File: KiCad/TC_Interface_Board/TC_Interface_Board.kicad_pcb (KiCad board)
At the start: 2 copper layers, 68.9 x 121.6 mm, 30 parts, among them J1 JST_VH_01x05, J1_24V1 JST_VH_01x04, J1_CN1 JST_VH_01x03, J2 JST_VH_01x05, J2_CN1 JST_VH_01x02, J3 JST_VH_01x05, J3_CN1 JST_VH_01x02, J4 JST_VH_01x05, J5 JST_VH_01x05, J6 JST_VH_01x05, J7 JST_VH_01x05, J8 JST_VH_01x05, Q1 DTC143E, Q2 DTC143E, U1 MC34063AP

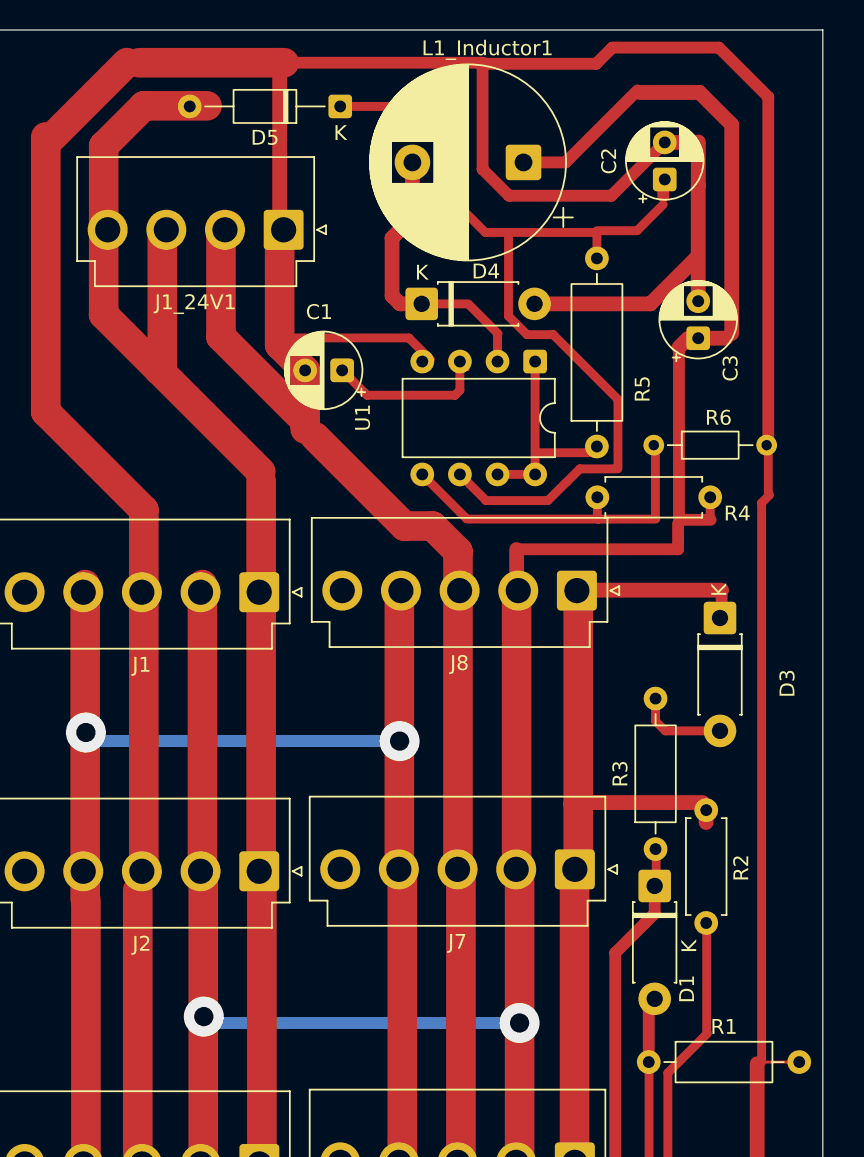
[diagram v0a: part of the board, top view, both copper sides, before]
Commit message: UPDATE
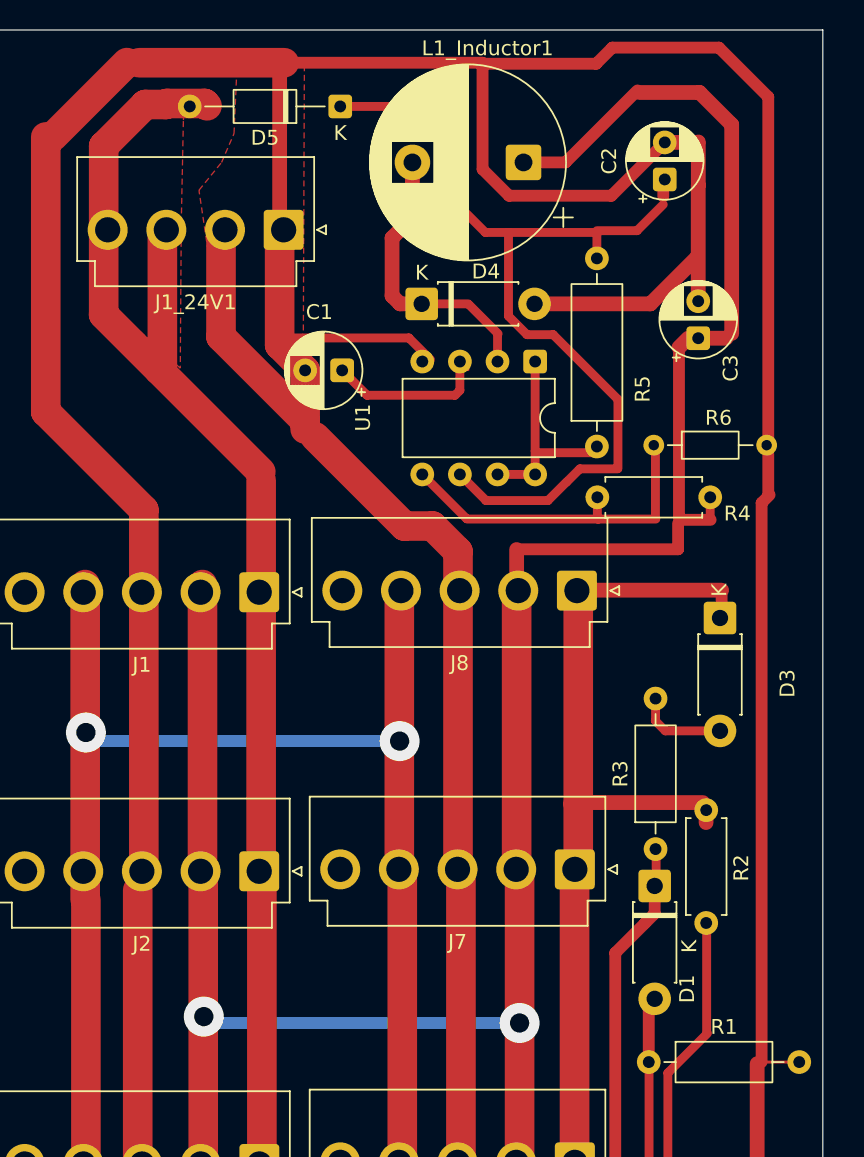
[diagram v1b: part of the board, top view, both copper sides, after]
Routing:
- added copper zone on F.Cu, net +24V
- added copper zone on F.Cu, net GND
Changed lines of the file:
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@@
+	)
+	(segment
+		(start 135.96 37.09)
+		(end 136.12 37.25)
+		(width 2)
+		(layer "F.Cu")
+		(net 1)
 	)
 	(segment
@@
 	)
 	(segment
+		(start 129.14 39.97)
+		(end 131.95 37.16)
+		(width 2)
+		(layer "F.Cu")
+		(net 1)
+	)
+	(segment
 		(start 169.81 85.64)
 		(end 169.81 84.51)
@@
 	)
 	(segment
-		(start 129.14 45.72)
-		(end 129.14 39.97)
-		(width 2)
-		(layer "F.Cu")
-		(net 1)
-	)
-	(segment
 		(start 161.2 69.95)
 		(end 160.98 70.17)
@@
 	)
 	(segment
-		(start 131.86 37.25)
-		(end 136.12 37.25)
+		(start 129.14 51.33)
+		(end 129.14 39.97)
+		(width 2)
+		(layer "F.Cu")
+		(net 1)
+	)
+	(segment
+		(start 133.41 37.09)
+		(end 135.96 37.09)
 		(width 2)
 		(layer "F.Cu")
@@
 	)
 	(segment
+		(start 131.95 37.16)
+		(end 133.34 37.16)
+		(width 2)
+		(layer "F.Cu")
+		(net 1)
+	)
+	(segment
+		(start 133.34 37.16)
+		(end 133.41 37.09)
+		(width 2)
+		(layer "F.Cu")
+		(net 1)
+	)
+	(segment
 		(start 139.77 62.54)
 		(end 139.75 62.52)
@@
 	)
 	(segment
-		(start 129.14 51.33)
-		(end 129.14 45.72)
-		(width 2)
-		(layer "F.Cu")
-		(net 1)
-	)
-	(segment
 		(start 132.87 55.08)
 		(end 129.13 51.34)
@@
 	)
 	(segment
-		(start 129.14 39.97)
-		(end 131.86 37.25)
-		(width 2)
-		(layer "F.Cu")
-		(net 1)
-	)
-	(segment
 		(start 161.096428 133.96)
 		(end 161.2 133.856428)
@@
 		(start 174.01 63.43)
 		(end 174.01 60.771)
-		(width 0.6)
+		(width 0.8)
 		(layer "F.Cu")
 		(net 4)
@@
 		(start 173.56 101.81)
 		(end 173.56 64.06)
-		(width 0.6)
+		(width 0.8)
 		(layer "F.Cu")
 		(net 4)
@@
 		(start 173.56 64.06)
 		(end 174.1 63.52)
-		(width 0.6)
+		(width 0.8)
 		(layer "F.Cu")
 		(net 4)
@@
 		(net 21)
 	)
+	(zone
+		(net 4)
+		(net_name "GND")
+		(layer "F.Cu")
+		(hatch edge 0.5)
+		(priority 1)
+		(connect_pads
+			(clearance 0.5)
+		)
+		(min_thickness 0.25)
+		(filled_areas_thickness no)
+		(fill yes
+			(thermal_gap 0.5)
+			(thermal_bridge_width 0.5)
+		)
+		(polygon
+			(pts
+				(xy 142.69 34.51) (xy 142.62 52.65) (xy 141.43 53.35) (xy 142.06 56.49) (xy 137.06 52.84) (xy 135.5725 42.95)
+				(xy 137.1 41.07) (xy 137.94 39.12) (xy 138.15 34.37) (xy 142.83 34.51)
+			)
+		)
+	)
+	(zone
+		(net 1)
+		(net_name "+24V")
+		(layer "F.Cu")
+		(hatch edge 0.5)
+		(connect_pads
+			(clearance 0.5)
+		)
+		(min_thickness 0.25)
+		(filled_areas_thickness no)
+		(fill yes
+			(thermal_gap 0.5)
+			(thermal_bridge_width 0.5)
+		)
+		(polygon
+			(pts
+				(xy 134.52 38.28) (xy 134.38 45.07) (xy 134.31 54.96) (xy 129.71 50.77) (xy 129.78 40.16) (xy 132.43 37.93)
+				(xy 134.59 37.16)
+			)
+		)
+	)
 	(embedded_fonts no)

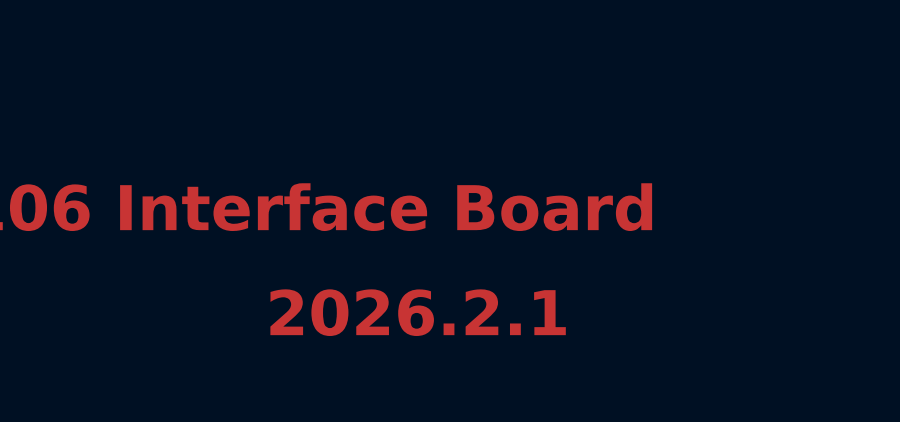
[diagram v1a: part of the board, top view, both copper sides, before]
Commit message: UPDATE
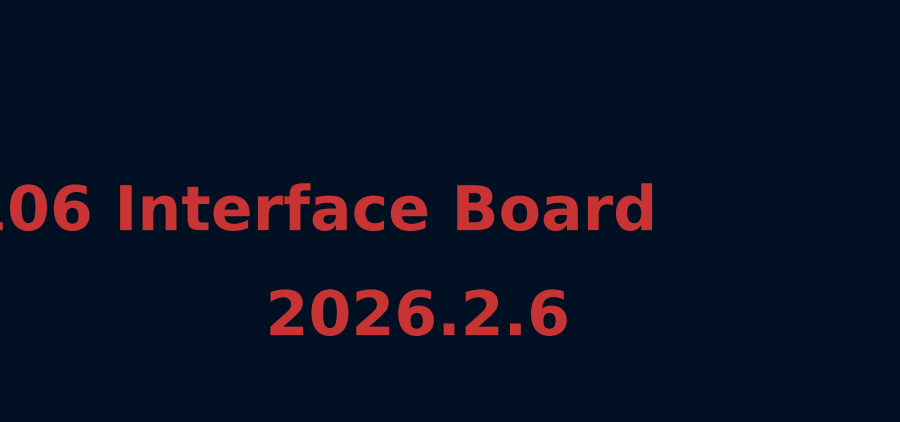
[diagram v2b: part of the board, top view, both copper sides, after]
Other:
- board text added: "2026.2.6"
- board text removed: "2026.2.1"
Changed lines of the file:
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@@
 		)
 	)
-	(gr_text "2026.2.1"
+	(gr_text "2026.2.6"
 		(at 212 194 0)
 		(layer "F.Cu")
